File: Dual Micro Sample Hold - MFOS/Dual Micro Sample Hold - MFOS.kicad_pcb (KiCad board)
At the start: 2 copper layers, 58.2 x 46.7 mm, 44 parts, among them J1 +12V_Conn, J10 TRIG_A, J11 CV_OUT_A, J12 GLIDE_OUT_A, J2 GND_Conn, J3 -12V_Conn, J4 IN_A, J5 SampRate_1W_A, J6 SampRate_3_A, J7 LED_A, J8 Glide_1W_A, J9 Glide_3_A, Q1 Q_NJFET_DSG, U1 LF444

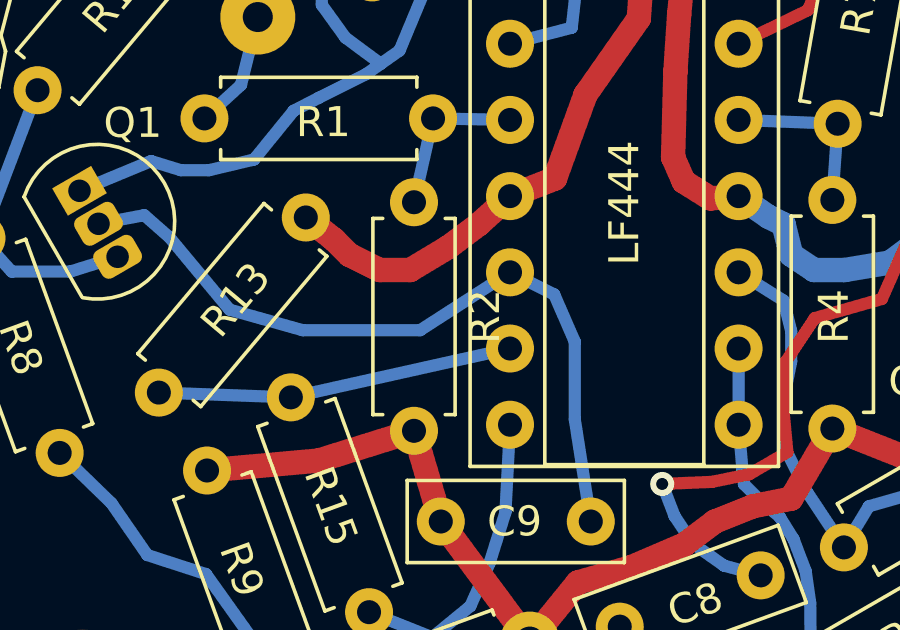
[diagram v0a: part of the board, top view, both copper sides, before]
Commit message: literally so much stuff
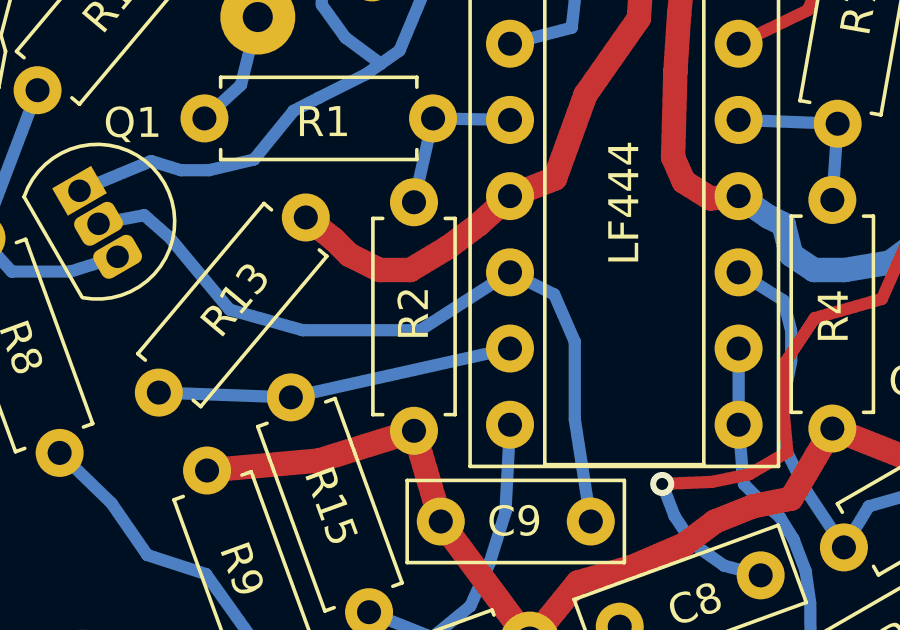
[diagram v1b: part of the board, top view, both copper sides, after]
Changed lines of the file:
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@@
     (descr "Resistor, Axial_DIN0207 series, Axial, Horizontal, pin pitch=7.62mm, 0.25W = 1/4W, length*diameter=6.3*2.5mm^2, http://cdn-reichelt.de/documents/datenblatt/B400/1_4W%23YAG.pdf")
     (tags "Resistor Axial_DIN0207 series Axial Horizontal pin pitch 7.62mm 0.25W = 1/4W length 6.3mm diameter 2.5mm")
-    (fp_text reference R2 (at 3.81 -2.37 90) (layer F.SilkS)
+    (fp_text reference R2 (at 3.7084 0 90) (layer F.SilkS)
       (effects (font (size 1 1) (thickness 0.15)))
     )
